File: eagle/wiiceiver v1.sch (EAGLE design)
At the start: 15 parts, among them IC1 ATmega328P, IC2 317T

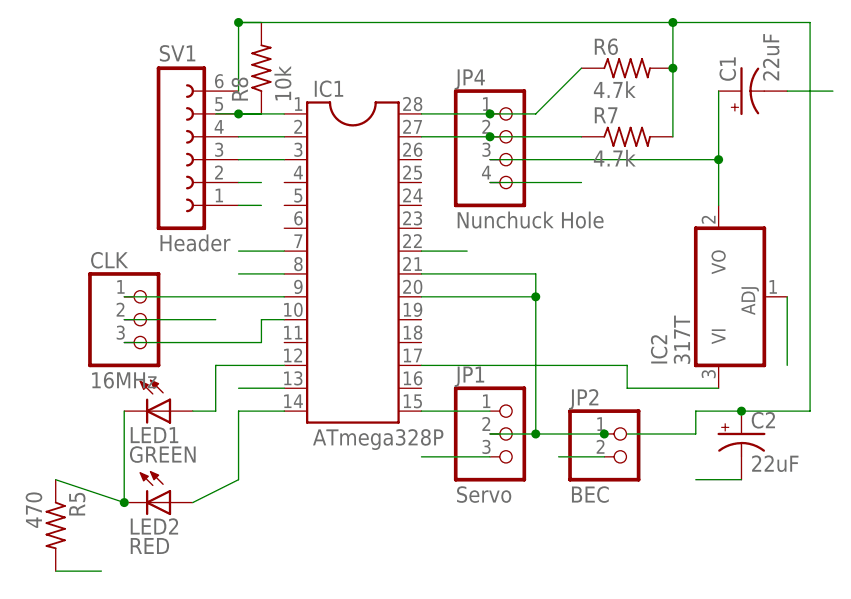
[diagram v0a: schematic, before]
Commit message: ordered!
“final” version, ordered from OshPark
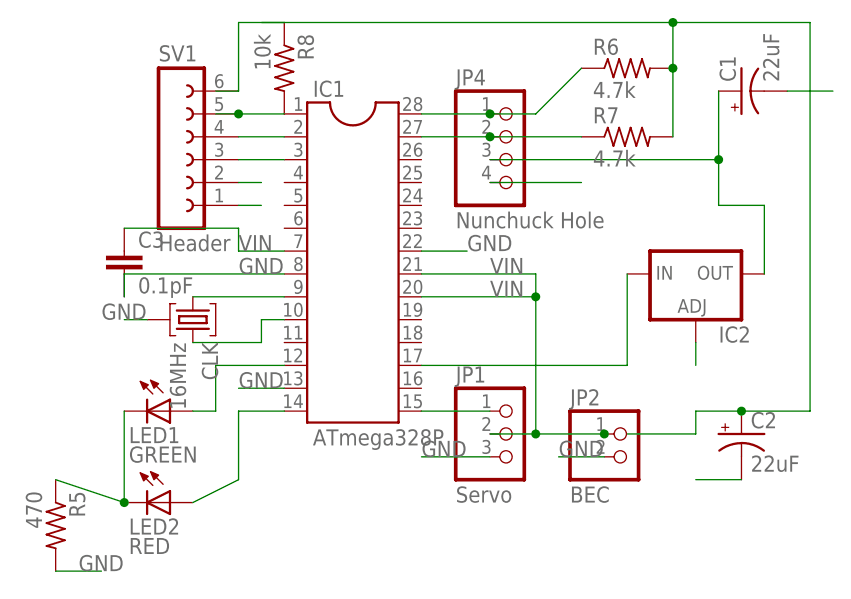
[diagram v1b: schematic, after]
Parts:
- added C3: 0.1pF, capacitor-wima:C5/2.5
- CLK: device pinhead:PINHD-1X3 -> crystal:IXFA
- IC1: device ic-package:DIL28 -> ic-package:DIL28-3
- IC2: value 317T -> (none); device linear:317T -> v-reg:LM317TS
- R5, R6, R7, R8: device rcl:R-US_0207/7 -> resistor:R-US_0204/2V
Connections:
- removed net N$12: IC1.1, R8.1, SV1.5
- new net N$2: IC1.1, R8.2, SV1.5
- net GND: now also C3.2
- net N$10: now also IC2.IN; no longer IC2.VI
- net N$16: now also IC2.OUT; no longer IC2.VO
- net VIN: now also C3.1, R8.1; no longer R8.2
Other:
- moved on the sheet: R8
